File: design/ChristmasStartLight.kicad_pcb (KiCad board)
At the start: 2 copper layers, 10 parts, among them P1 CONN_2, Q1 MPS2222A, U1 TCL555CP

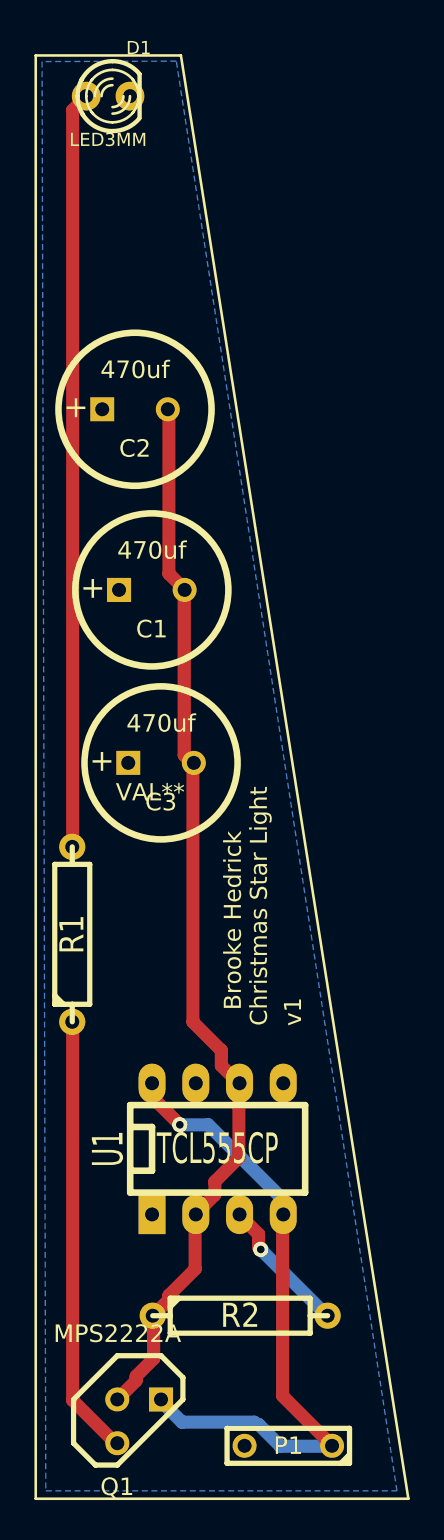
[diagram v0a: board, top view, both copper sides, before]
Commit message: Parts and PCB done
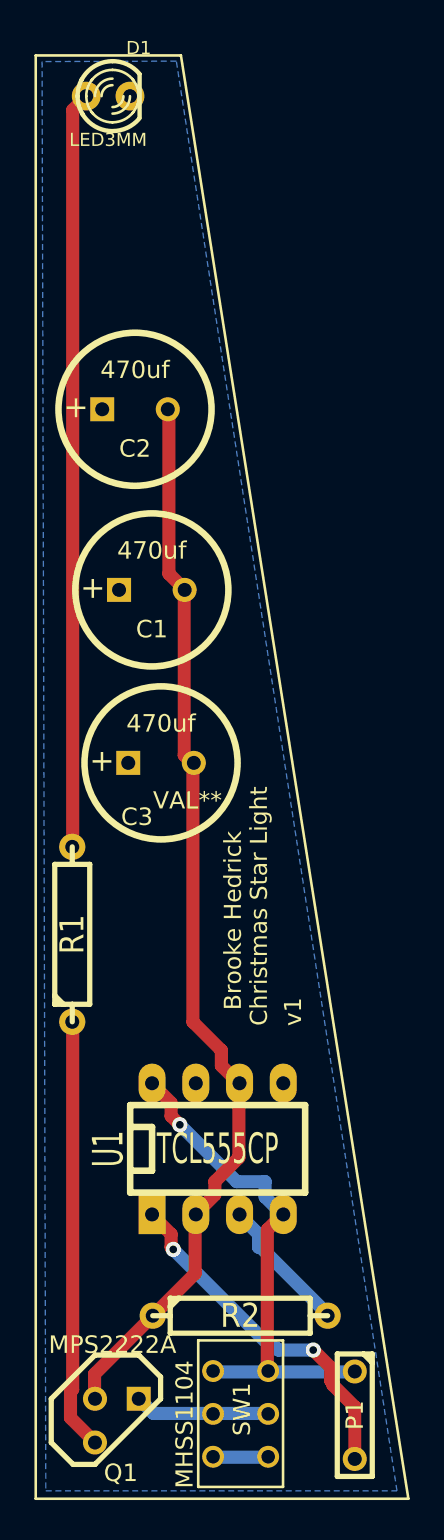
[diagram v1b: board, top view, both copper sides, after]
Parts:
- added SW1: MHSS1104, MHSS1104_MICROSWITCH_SPDT, F.Cu at (135.5, 131.5)
- moved P1 4.25 mm to (142.1, 131.7), turned to 270 degrees
- moved Q1 1.30 mm to (128.3, 132.0)
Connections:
- Q1 pad 1: VCC -> N-000005
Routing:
- net GND: track 0.00 -> 20.5 mm, vias 0 -> 2
- net N-000005: track 0.00 -> 8.04 mm
- net VCC: track 37.8 -> 29.9 mm
- net N-000008: track 0.00 -> 3.27 mm
- net N-0000010: track 62.7 -> 63.2 mm
- net N-000004: track 25.6 -> 25.1 mm
- net N-000003: vias 1 -> 0
